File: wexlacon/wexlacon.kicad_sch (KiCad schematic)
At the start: 13 parts, among them J1 MVE252-5-V, J10 solder, J3 KK-254, J5 CAN25, J6 pinheader, J9 MVE253-5-V

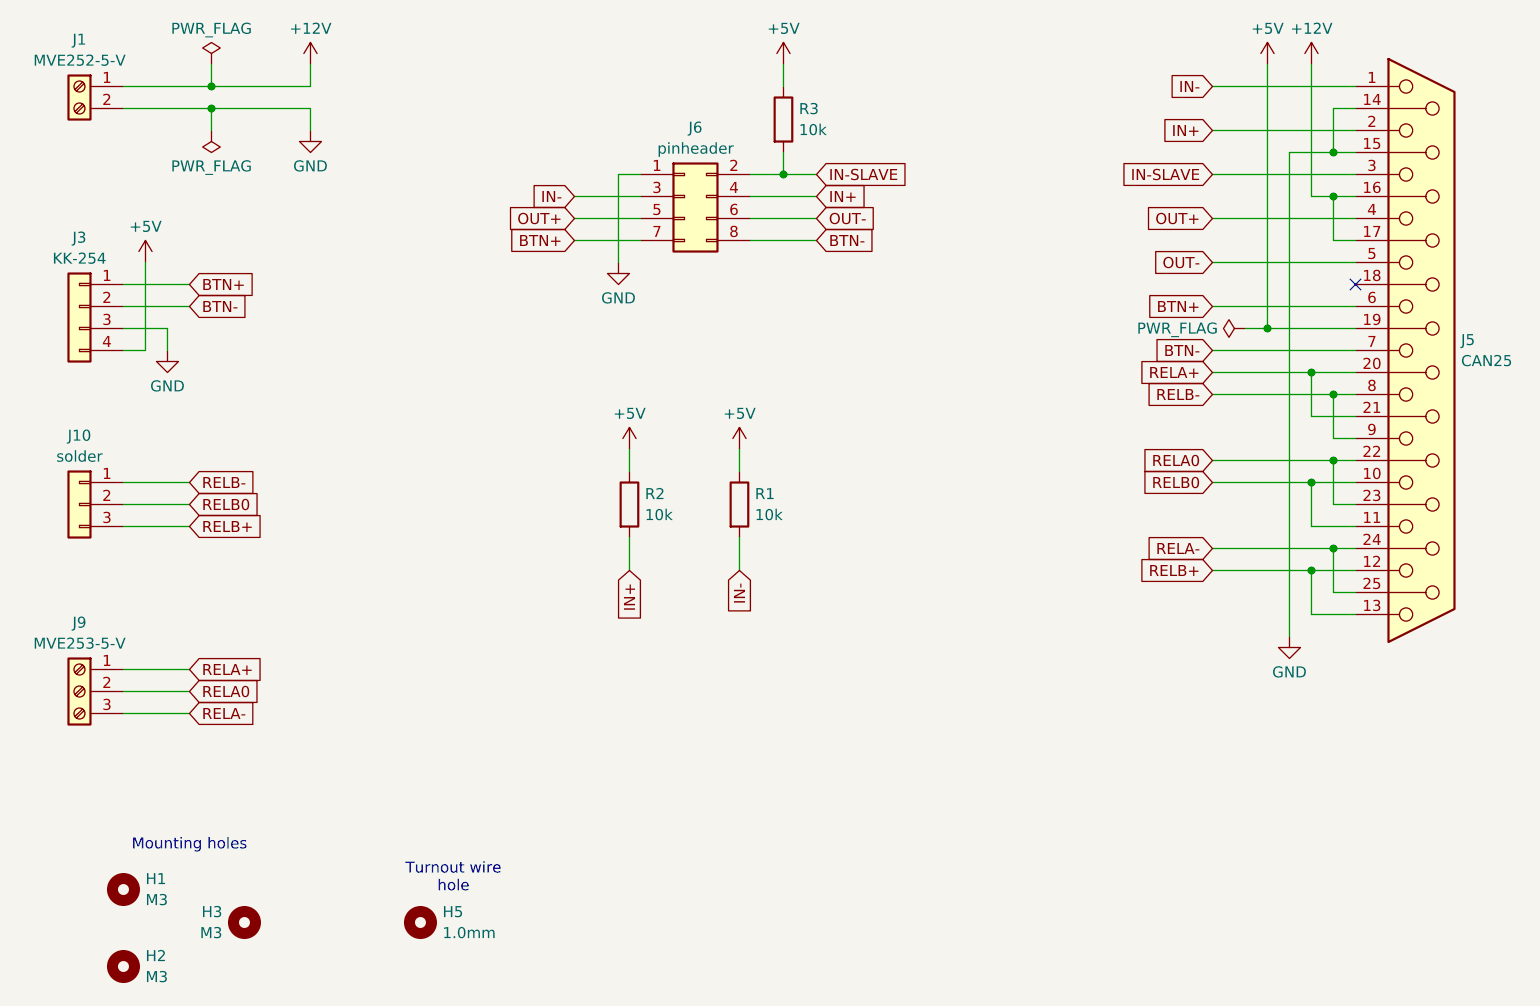
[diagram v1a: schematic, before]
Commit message: Fix switched order of relay contacts.
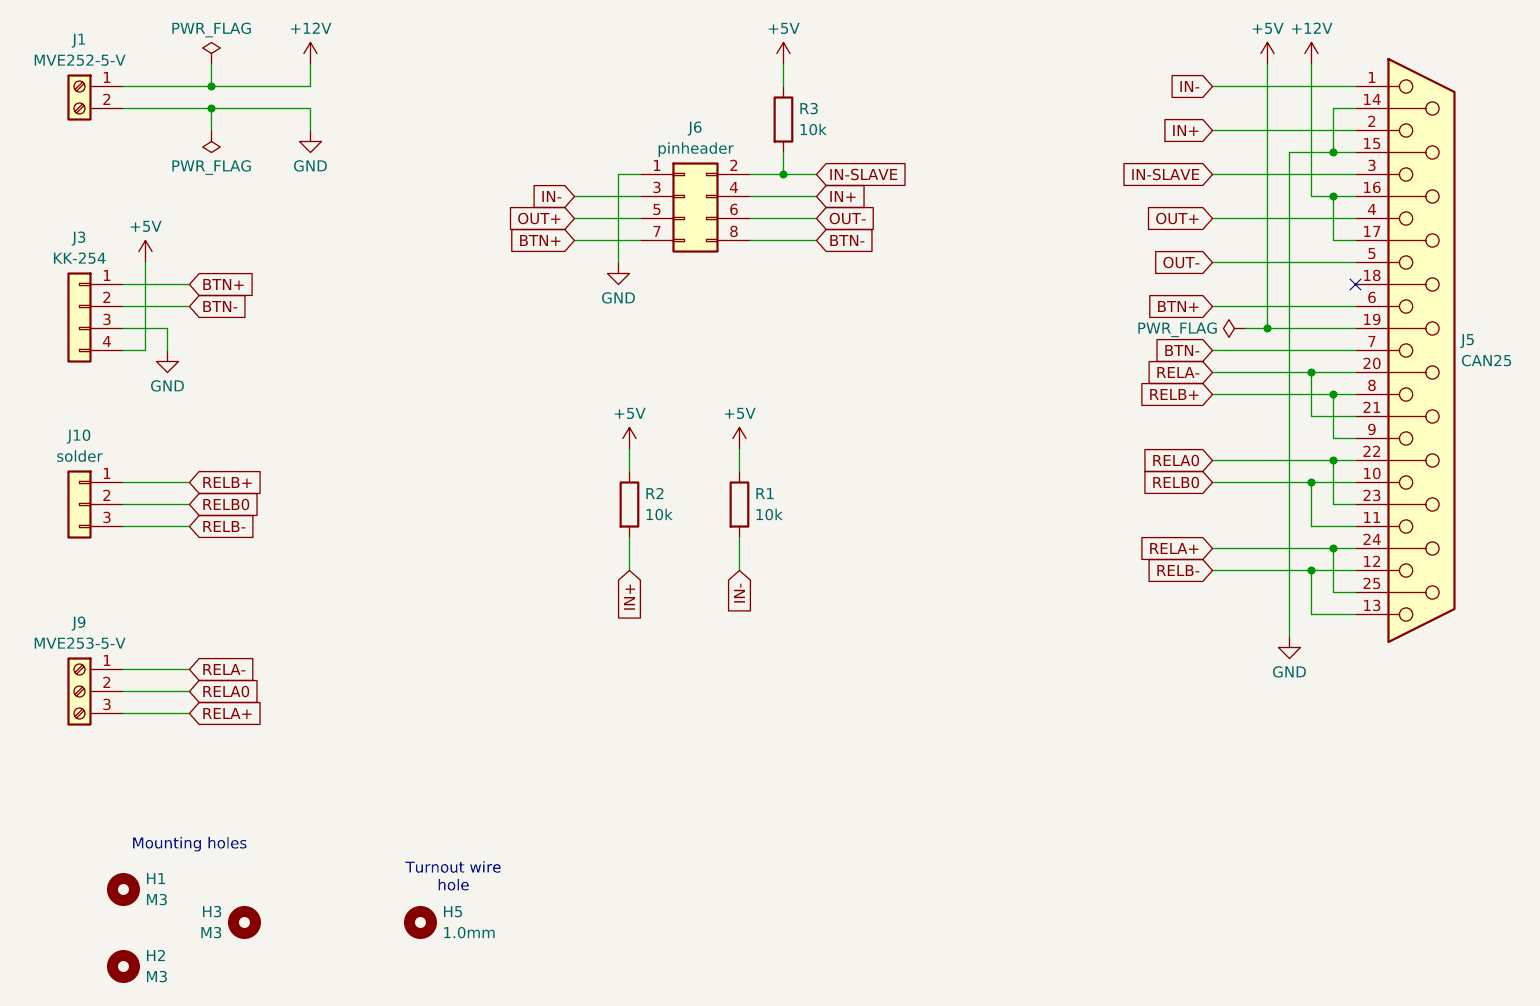
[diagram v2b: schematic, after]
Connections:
- net RELA+: now also J5.24 (P24), J5.25 (P25), J9.3 (Pin_3); no longer J5.20 (P20), J5.21 (P21), J9.1 (Pin_1)
- net RELA-: now also J5.20 (P20), J5.21 (P21), J9.1 (Pin_1); no longer J5.24 (P24), J5.25 (P25), J9.3 (Pin_3)
- net RELB+: now also J10.1 (Pin_1), J5.8, J5.9; no longer J10.3 (Pin_3), J5.12, J5.13
- net RELB-: now also J10.3 (Pin_3), J5.12, J5.13; no longer J10.1 (Pin_1), J5.8, J5.9
